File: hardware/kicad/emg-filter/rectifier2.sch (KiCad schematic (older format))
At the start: 80 parts

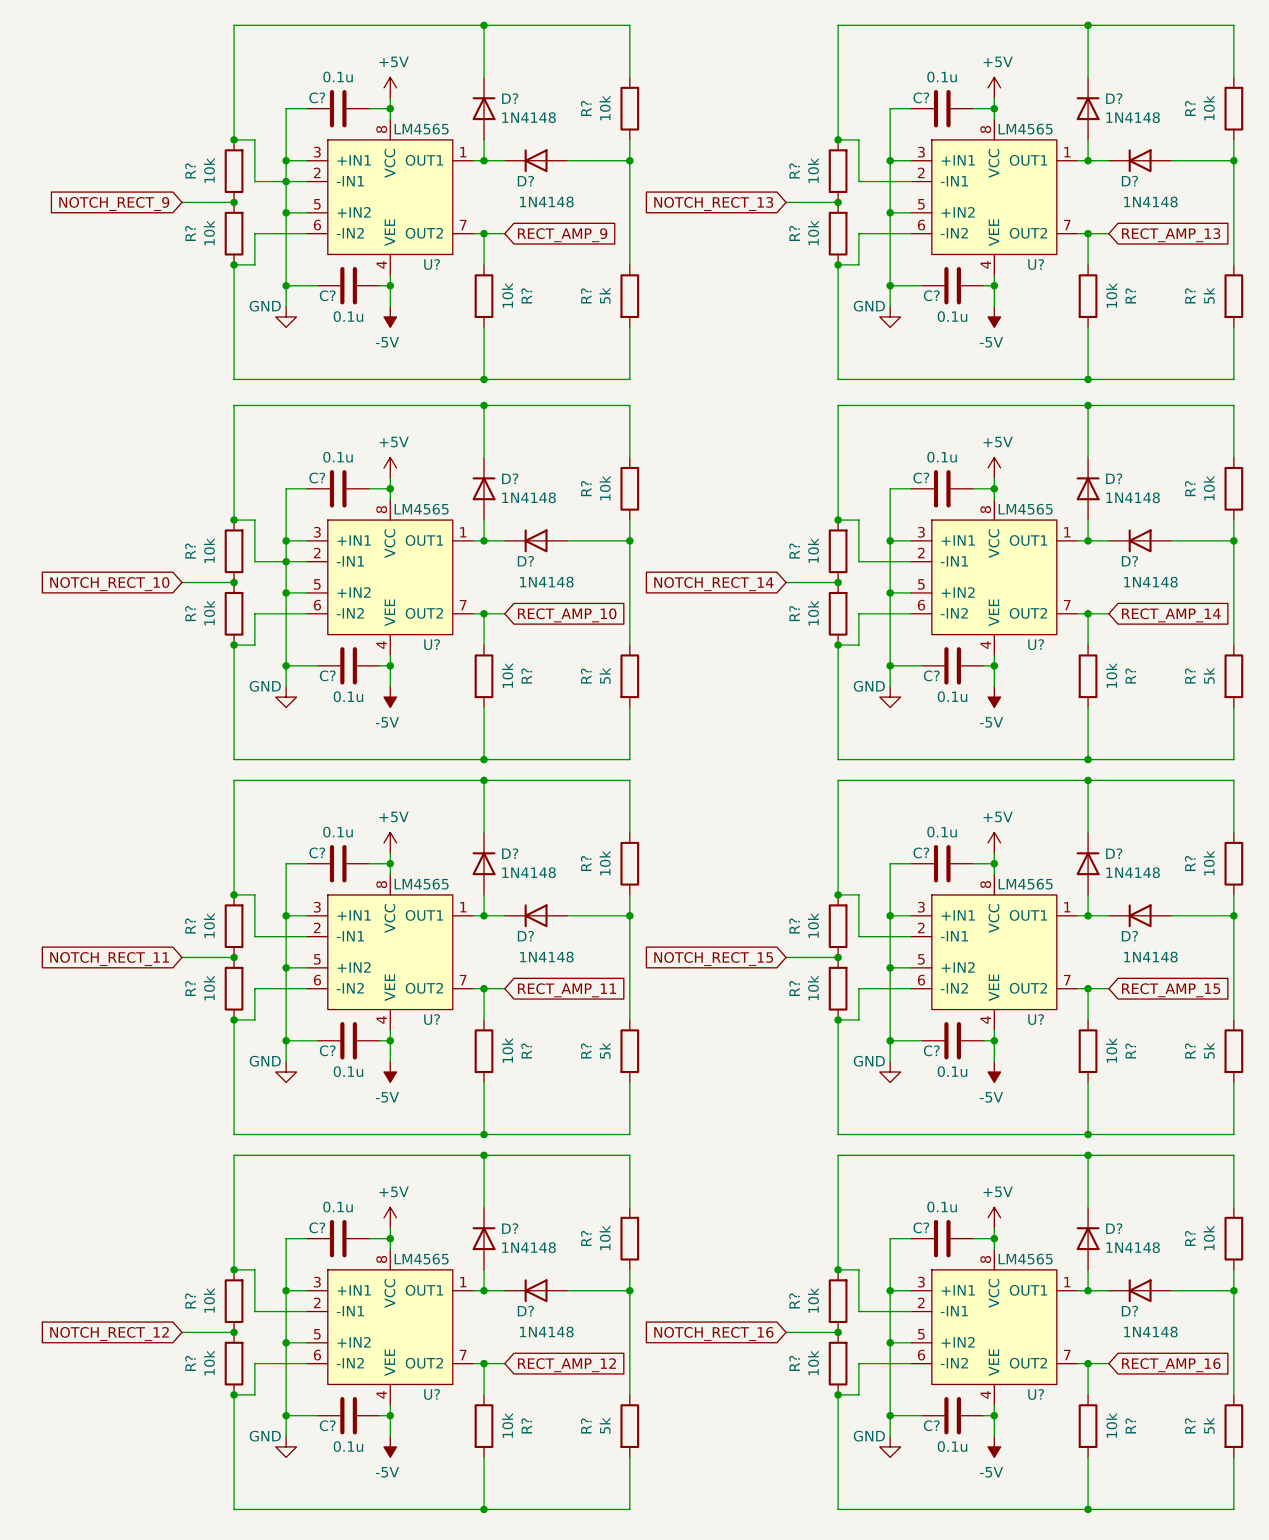
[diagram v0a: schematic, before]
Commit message: Connector
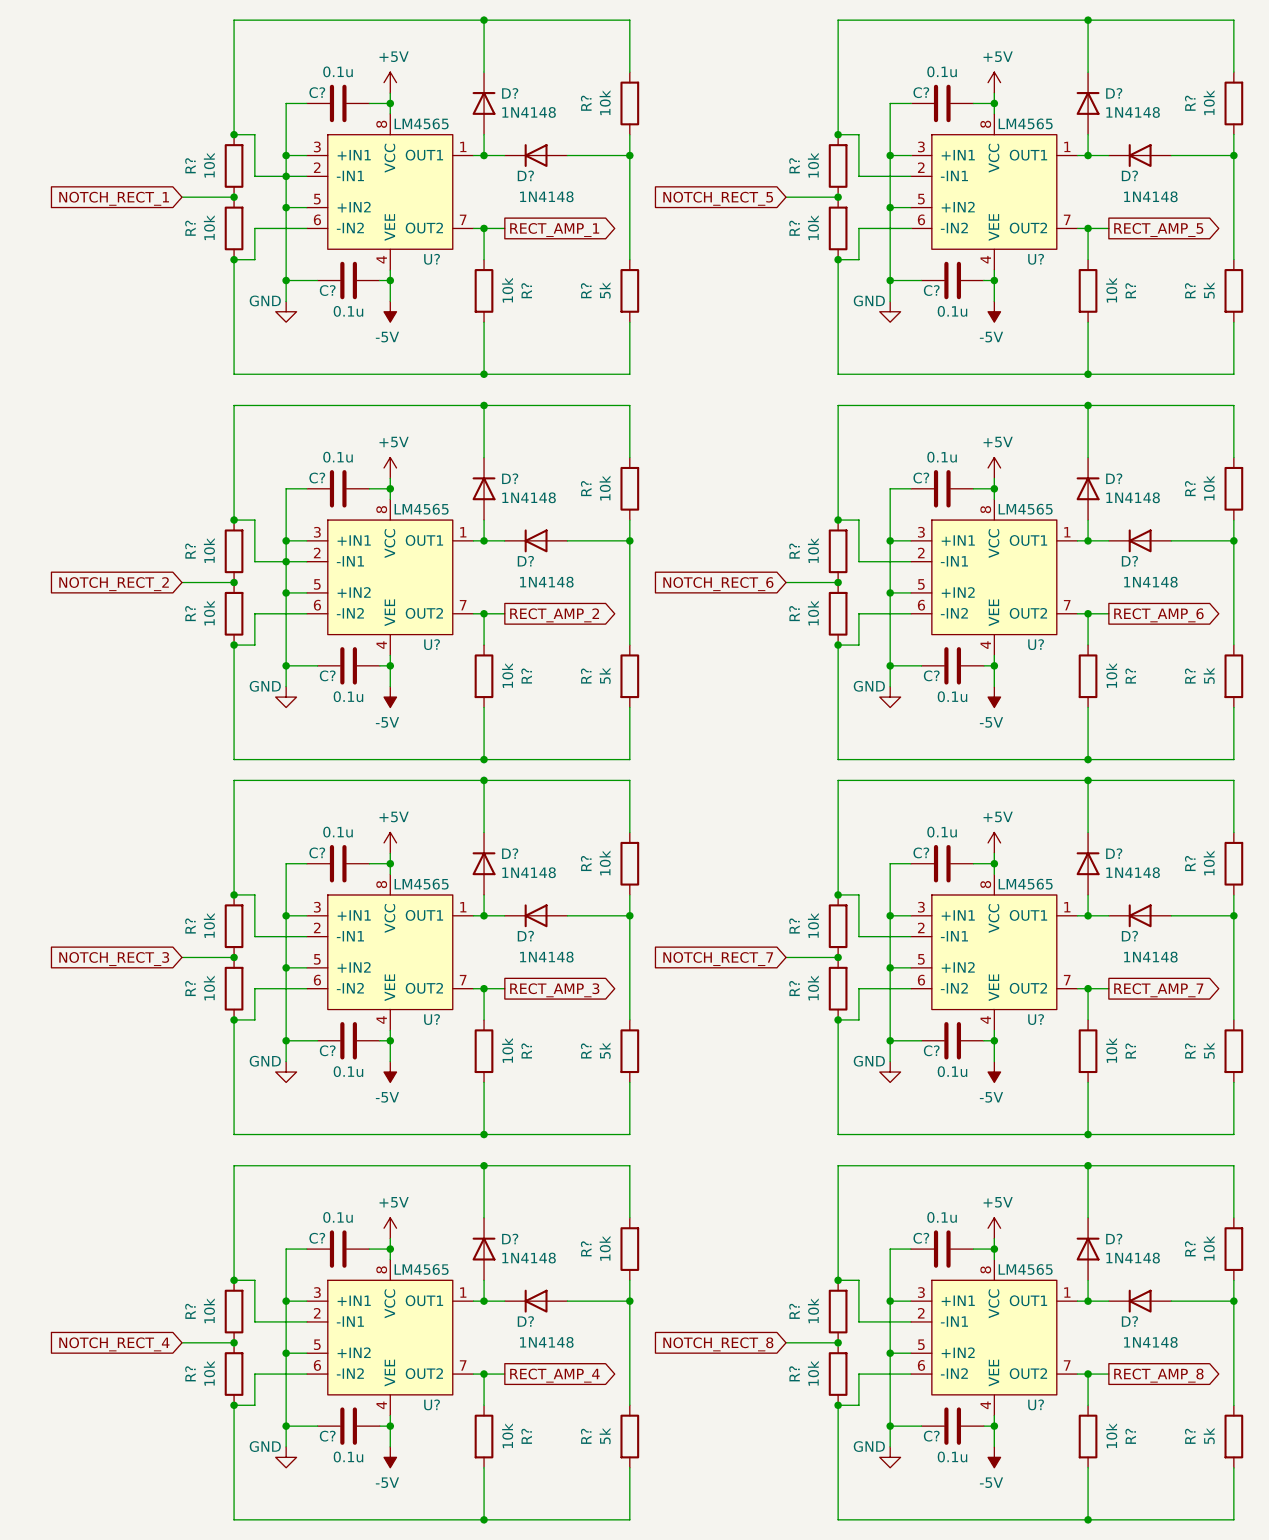
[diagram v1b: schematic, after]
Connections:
- net NOTCH_RECT_10 renamed NOTCH_RECT_2
- net NOTCH_RECT_11 renamed NOTCH_RECT_3
- net NOTCH_RECT_12 renamed NOTCH_RECT_4
- net NOTCH_RECT_13 renamed NOTCH_RECT_5
- net NOTCH_RECT_14 renamed NOTCH_RECT_6
- net NOTCH_RECT_15 renamed NOTCH_RECT_7
- net NOTCH_RECT_16 renamed NOTCH_RECT_8
- net NOTCH_RECT_9 renamed NOTCH_RECT_1
- net RECT_AMP_10 renamed RECT_AMP_2
- net RECT_AMP_11 renamed RECT_AMP_3
- net RECT_AMP_12 renamed RECT_AMP_4
- net RECT_AMP_13 renamed RECT_AMP_5
- net RECT_AMP_14 renamed RECT_AMP_6
- net RECT_AMP_15 renamed RECT_AMP_7
- net RECT_AMP_16 renamed RECT_AMP_8
- net RECT_AMP_9 renamed RECT_AMP_1
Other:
- moved on the sheet: C?, D?, R?, U?

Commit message: fixed rectifier
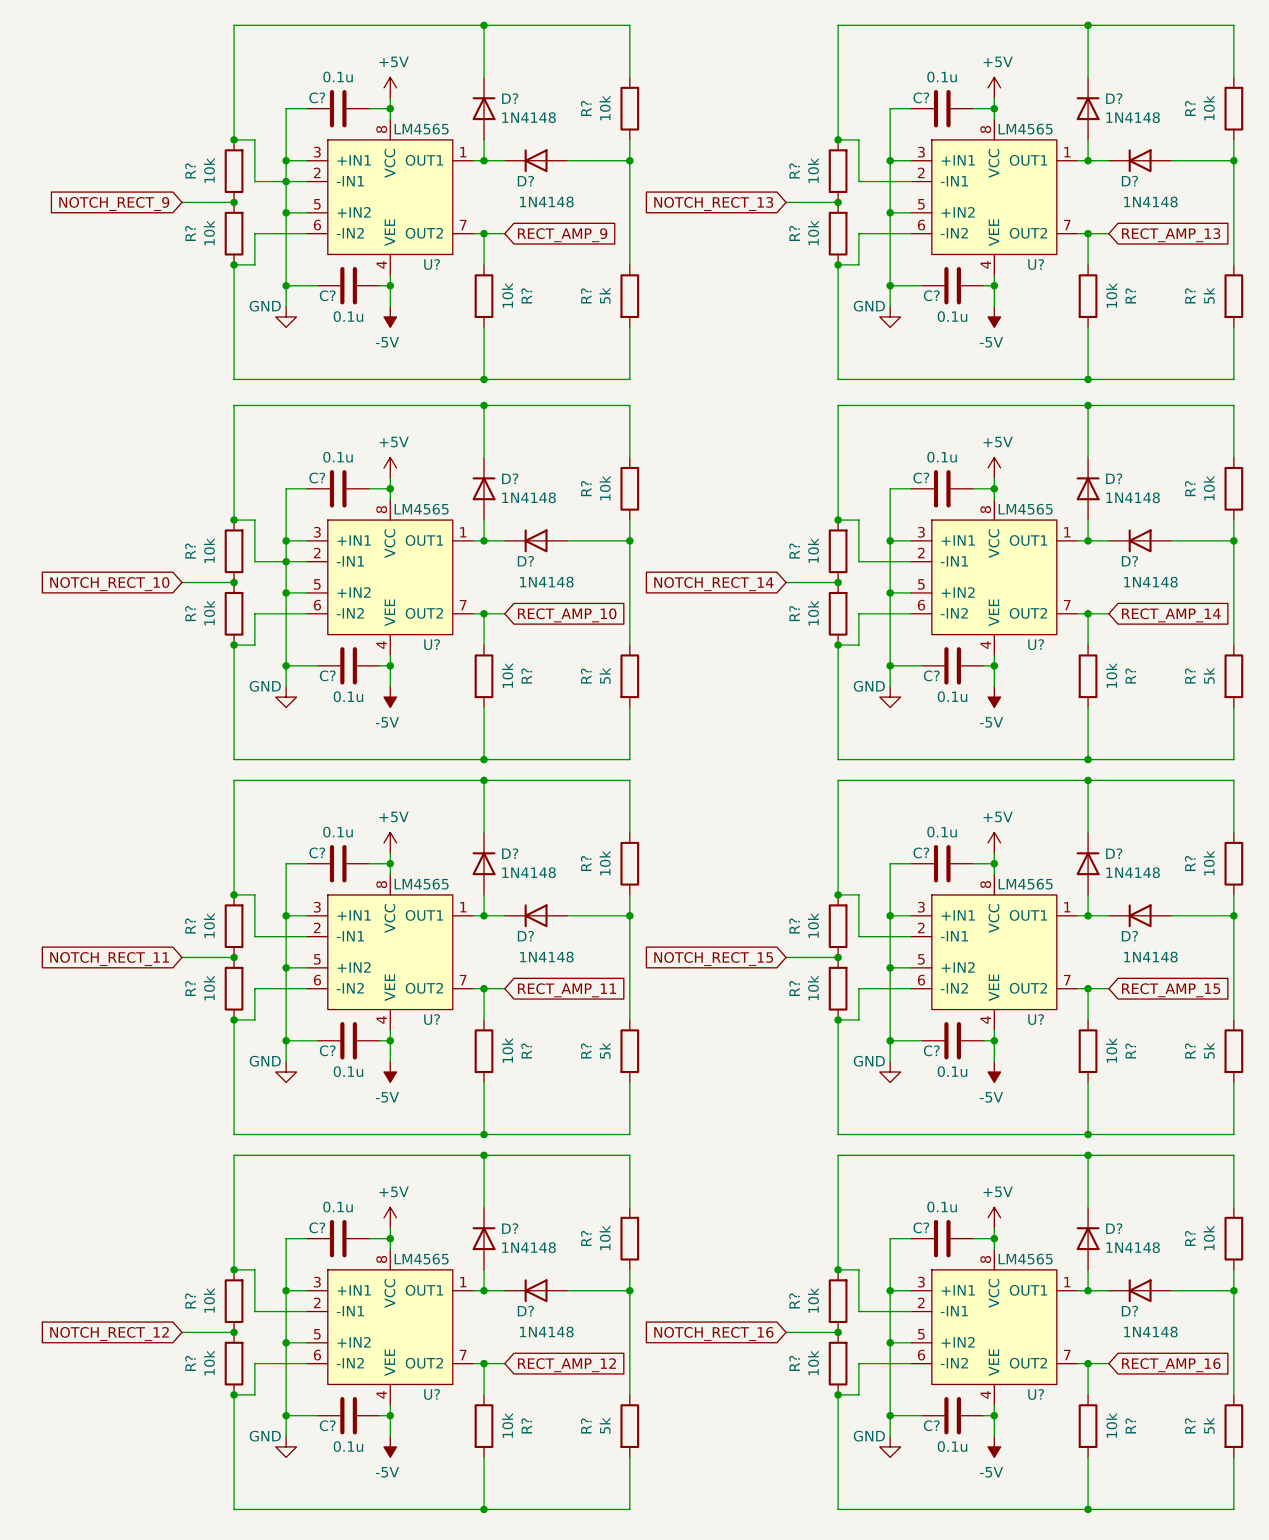
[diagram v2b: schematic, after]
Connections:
- net NOTCH_RECT_1 renamed NOTCH_RECT_9
- net NOTCH_RECT_2 renamed NOTCH_RECT_10
- net NOTCH_RECT_3 renamed NOTCH_RECT_11
- net NOTCH_RECT_4 renamed NOTCH_RECT_12
- net NOTCH_RECT_5 renamed NOTCH_RECT_13
- net NOTCH_RECT_6 renamed NOTCH_RECT_14
- net NOTCH_RECT_7 renamed NOTCH_RECT_15
- net NOTCH_RECT_8 renamed NOTCH_RECT_16
- net RECT_AMP_1 renamed RECT_AMP_9
- net RECT_AMP_2 renamed RECT_AMP_10
- net RECT_AMP_3 renamed RECT_AMP_11
- net RECT_AMP_4 renamed RECT_AMP_12
- net RECT_AMP_5 renamed RECT_AMP_13
- net RECT_AMP_6 renamed RECT_AMP_14
- net RECT_AMP_7 renamed RECT_AMP_15
- net RECT_AMP_8 renamed RECT_AMP_16
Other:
- moved on the sheet: C?, D?, R?, U?
